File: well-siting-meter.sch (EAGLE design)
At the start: 47 parts, among them J2 7805, T1 MOSFET-NCHANNELFQP30N06L, U1 LCD-16X2NOHOLES, U2 ARDUINO_PRO_MINI, U3 EC2, U4 EC2, U5 AD623, U6 AD623, U7 MAX1771

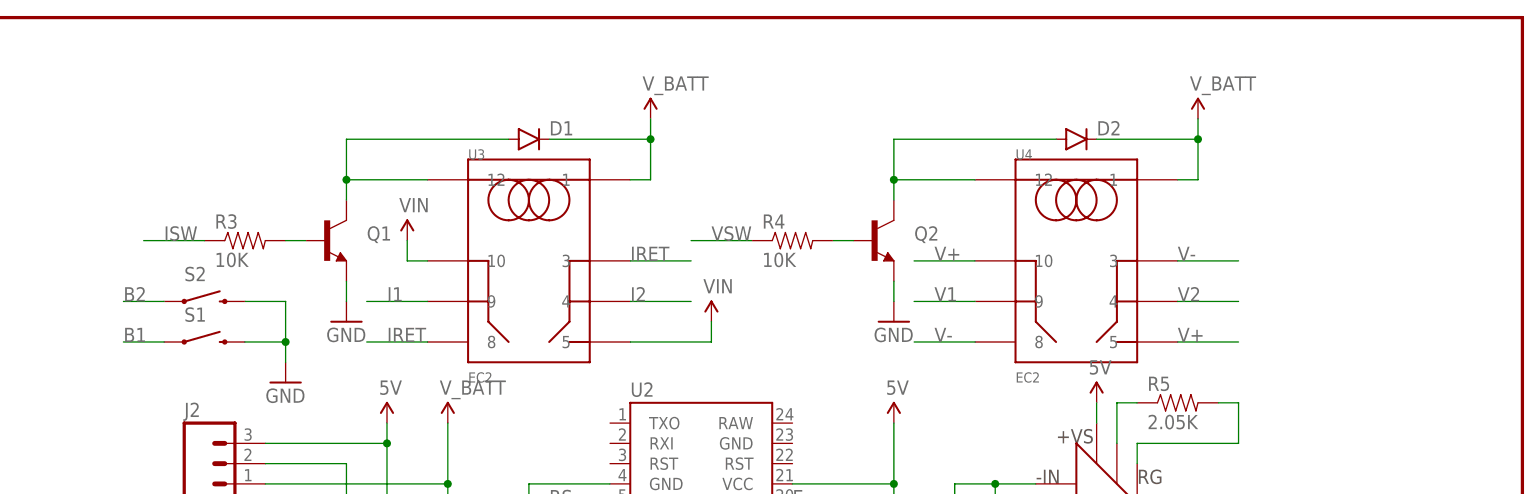
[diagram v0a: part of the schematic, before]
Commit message: rev A updates, arduino testing
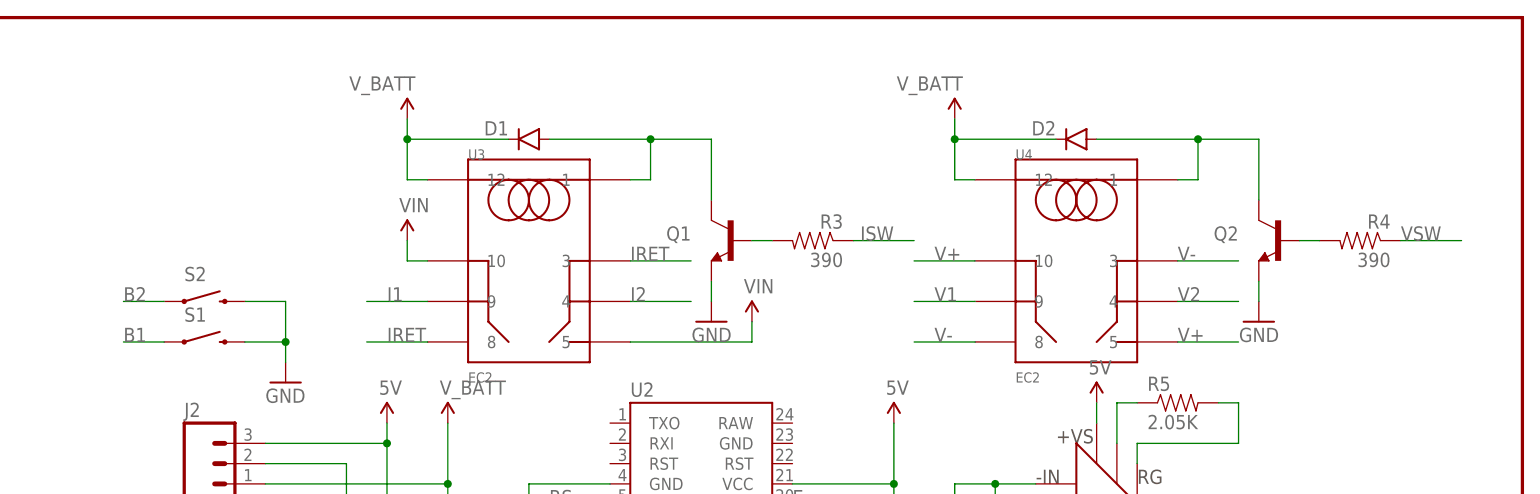
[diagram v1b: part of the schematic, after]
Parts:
- C1, C4: device SparkFun-Passives:CAP_POLPTH1 -> SparkFun-Passives:CAP_POLPTH4
- Q1, Q2: device SparkFun-DiscreteSemi:TRANSISTOR_NPNP2N2222A -> SparkFun-DiscreteSemi:TRANSISTOR_NPNTO92
- R3, R4: value 10K -> 390
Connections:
- net N$1: now also U4.1; no longer U4.12
- net N$4: now also U3.1; no longer U3.12
- net V_BATT: now also U3.12, U4.12; no longer U3.1, U4.1
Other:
- moved on the sheet: Q1, Q2, R3, R4
